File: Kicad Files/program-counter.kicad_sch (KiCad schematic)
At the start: 20 parts, among them U23 74LS161, U24 74LS161, U25 74LS245

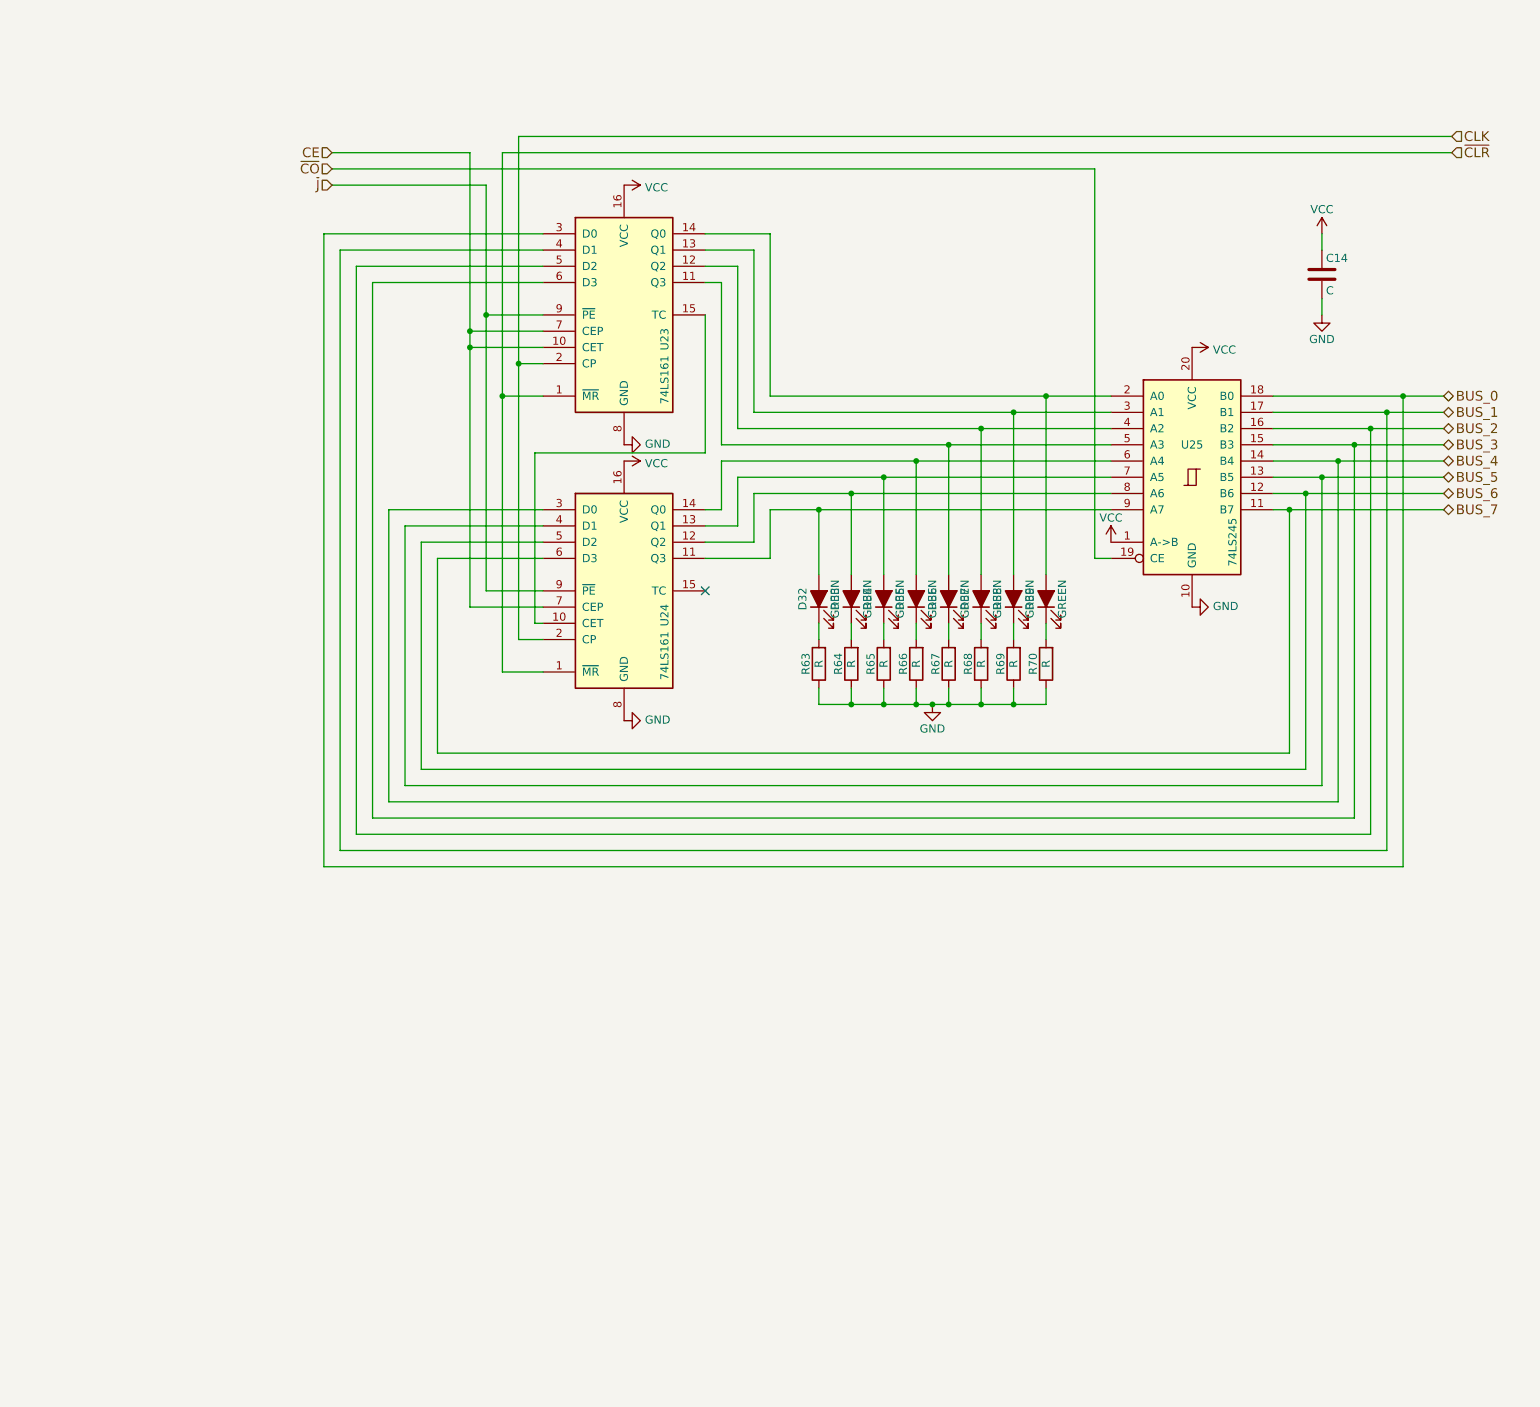
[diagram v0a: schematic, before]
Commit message: w2
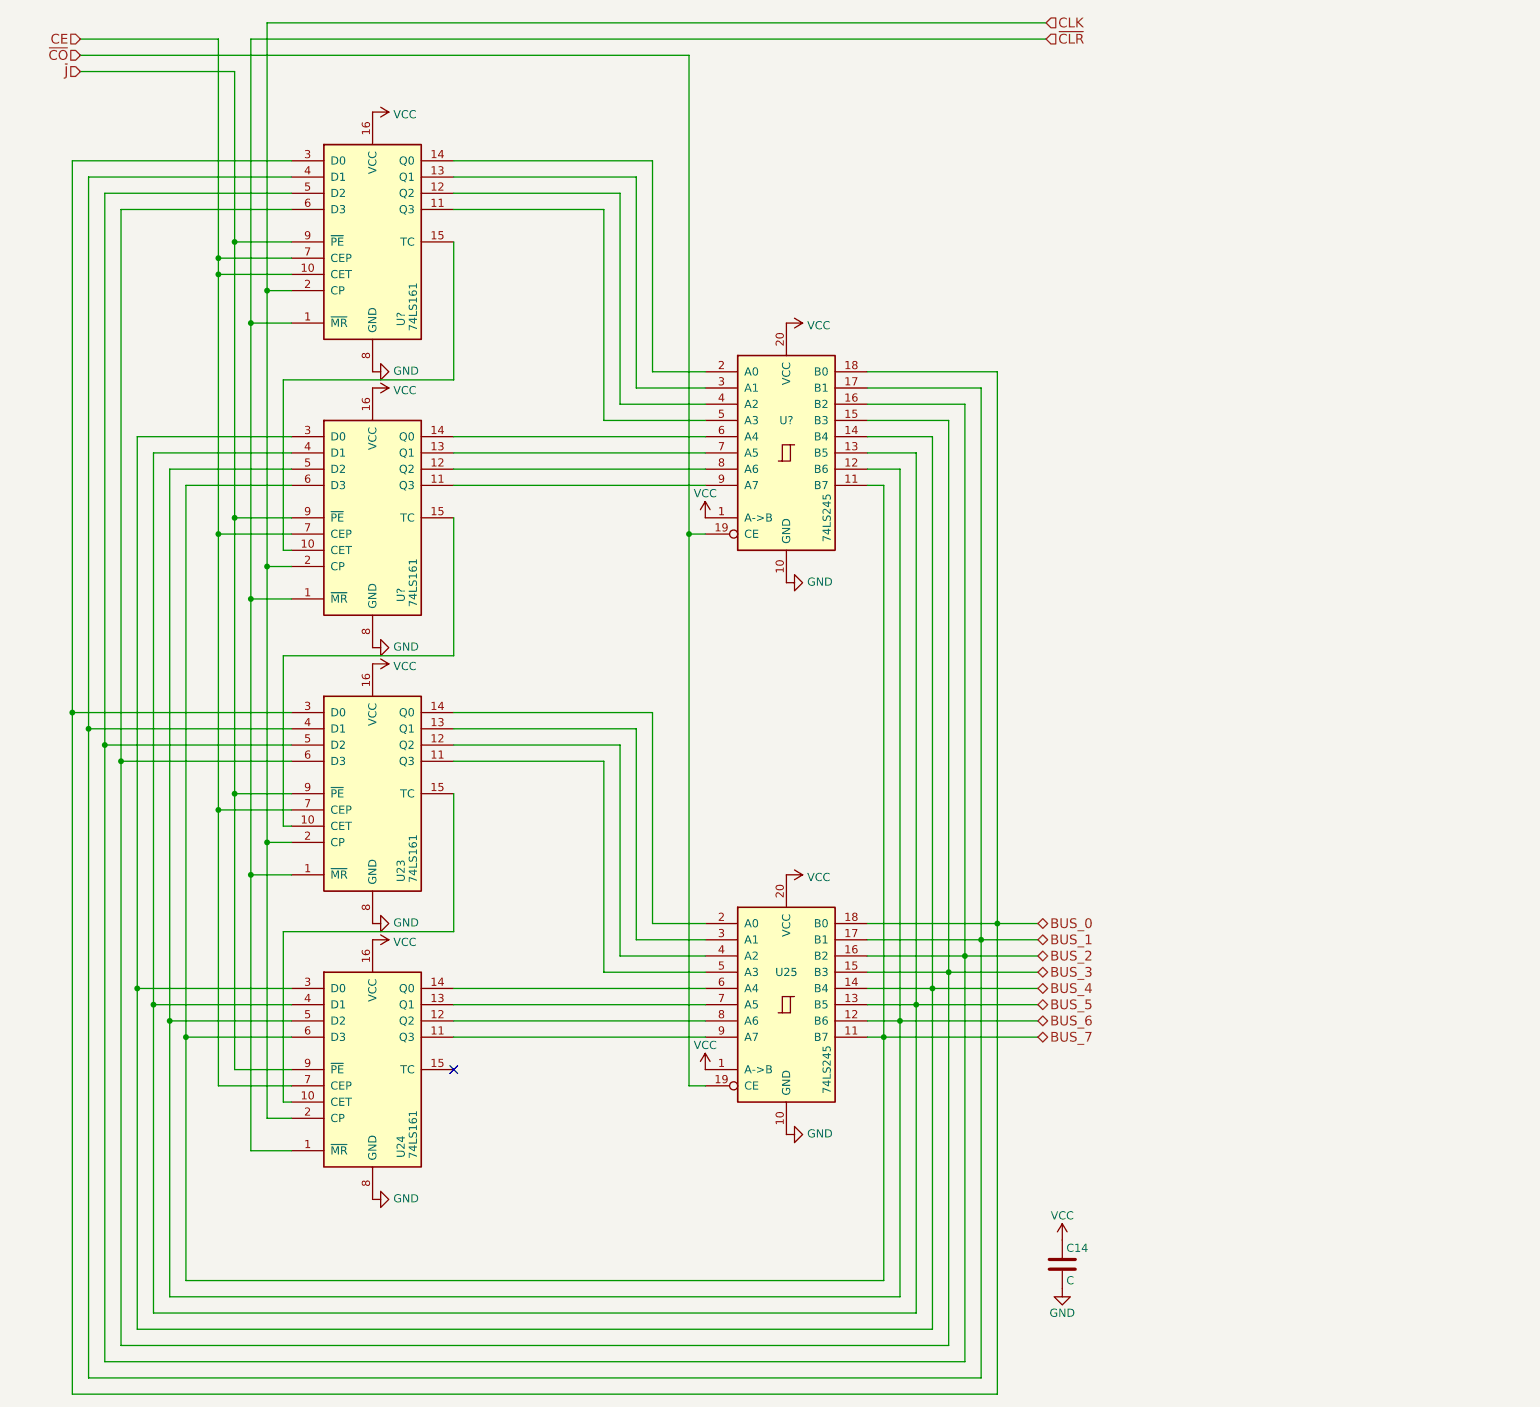
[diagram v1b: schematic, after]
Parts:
- removed D32, D33, D34, D35, D36, D37, D38, D39: GREEN, LED_THT:LED_D5.0mm, symbol 8bit-computer-rescue:LED_ALT-Device
- removed R63, R64, R65, R66, R67, R68, R69, R70: R, Resistor_THT:R_Axial_DIN0207_L6.3mm_D2.5mm_P7.62mm_Horizontal, symbol Device:R
- added U? (x2): 74LS161, symbol 74xx:74LS161
- added U?: 74LS245, symbol 74xx:74LS245
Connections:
- net BUS_0: now also U?.18 (B0), U?.3 (D0)
- net BUS_1: now also U?.17 (B1), U?.4 (D1)
- net BUS_2: now also U?.16 (B2), U?.5 (D2)
- net BUS_3: now also U?.15 (B3), U?.6 (D3)
- net BUS_4: now also U?.14 (B4), U?.3 (D0)
- net BUS_5: now also U?.13 (B5), U?.4 (D1)
- net BUS_6: now also U?.12 (B6), U?.5 (D2)
- net BUS_7: now also U?.11 (B7), U?.6 (D3)
- net CE: now also U?.10 (CET), U?.7 (CEP), U?.7 (CEP); no longer U23.10 (CET)
- net CLK: now also U?.2 (CP), U?.2 (CP)
- net GND: now also U?.10 (GND), U?.8 (GND), U?.8 (GND)
- net VCC: now also U?.1 (A->B), U?.16 (VCC), U?.16 (VCC), U?.20 (VCC)
- net ~{CLR}: now also U?.1 (~{MR}), U?.1 (~{MR})
- net ~{CO}: now also U?.19 (CE)
- net ~{J}: now also U?.9 (~{PE}), U?.9 (~{PE})
- new net: U23.10 (CET), U?.15 (TC)
- new net: U?.10 (CET), U?.15 (TC)
- new net: U?.11 (Q3), U?.9 (A7)
- new net: U?.12 (Q2), U?.8 (A6)
- new net: U?.13 (Q1), U?.7 (A5)
- new net: U?.14 (Q0), U?.6 (A4)
- new net: U?.11 (Q3), U?.5 (A3)
- new net: U?.12 (Q2), U?.4 (A2)
- new net: U?.13 (Q1), U?.3 (A1)
- new net: U?.14 (Q0), U?.2 (A0)
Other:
- moved on the sheet: C14, U23, U24, U25
